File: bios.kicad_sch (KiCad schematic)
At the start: 41 parts, among them J1201 Socket_SOP2-16_ACA-SPI-006-K0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, J1202 Socket_SOP2-16_ACA-SPI-006-K0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, U12 TMUX1574RSVR, U13 MT25QU01GBBB8_SOIC, U14 TMUX1574RSVR, U15 MT25QU01GBBB8_SOIC

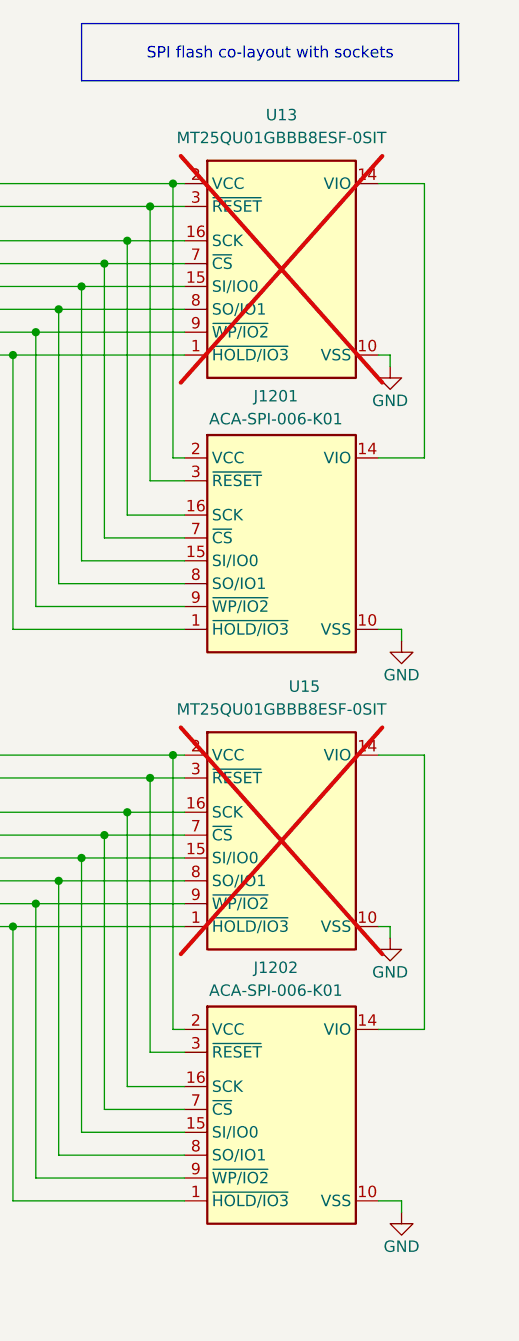
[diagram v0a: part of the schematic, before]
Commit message: [#101340] Add comments to ERC/DRC exclusions
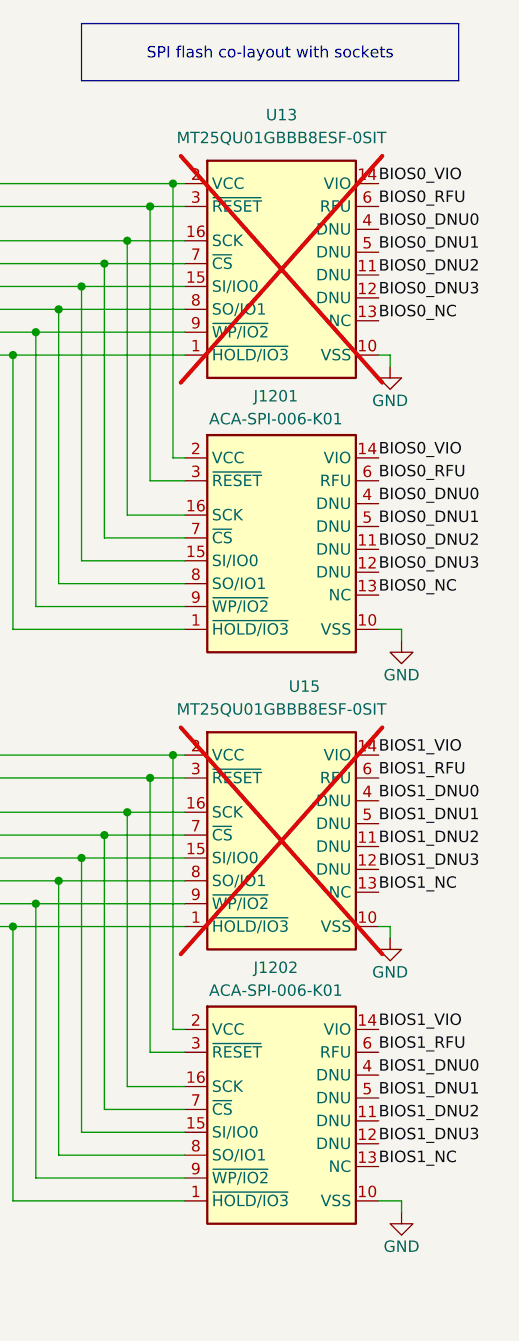
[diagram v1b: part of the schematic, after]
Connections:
- net BIOS1_NC: now reaches U15.13 (NC)
- net BIOS1_NC: now also J1202.13 (NC)
- net BIOS1_VIO: now reaches J1202.14 (VIO), U15.14 (VIO)
- net BIOS1_RFU: now reaches U15.6 (RFU)
- net BIOS1_RFU: now also J1202.6 (RFU)
- net BIOS0_NC: now reaches U13.13 (NC)
- net BIOS0_NC: now also J1201.13 (NC)
- net BIOS0_VIO: now reaches J1201.14 (VIO), U13.14 (VIO)
- net BIOS0_RFU: now reaches U13.6 (RFU)
- net BIOS0_RFU: now also J1201.6 (RFU)
- net BIOS0_DNU2: now reaches J1201.11 (DNU)
- net BIOS0_DNU2: now also U13.11 (DNU)
- net BIOS0_DNU3: now reaches J1201.12 (DNU)
- net BIOS0_DNU3: now also U13.12 (DNU)
- net BIOS0_DNU0: now reaches J1201.4 (DNU)
- net BIOS0_DNU0: now also U13.4 (DNU)
- net BIOS0_DNU1: now reaches J1201.5 (DNU)
- net BIOS0_DNU1: now also U13.5 (DNU)
- net BIOS1_DNU2: now reaches J1202.11 (DNU)
- net BIOS1_DNU2: now also U15.11 (DNU)
- net BIOS1_DNU3: now reaches J1202.12 (DNU)
- net BIOS1_DNU3: now also U15.12 (DNU)
- net BIOS1_DNU0: now reaches J1202.4 (DNU)
- net BIOS1_DNU0: now also U15.4 (DNU)
- net BIOS1_DNU1: now reaches J1202.5 (DNU)
- net BIOS1_DNU1: now also U15.5 (DNU)
